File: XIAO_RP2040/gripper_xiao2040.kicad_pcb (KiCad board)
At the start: 2 copper layers, 41 x 48 mm, 18 parts, among them J1 GoFa IO, J2 VGoFa, J3 Servo, J4 Magnet, J5 Conn_01x04, U1 XIAO-RP2040-DIP, U2 HCPL-2631

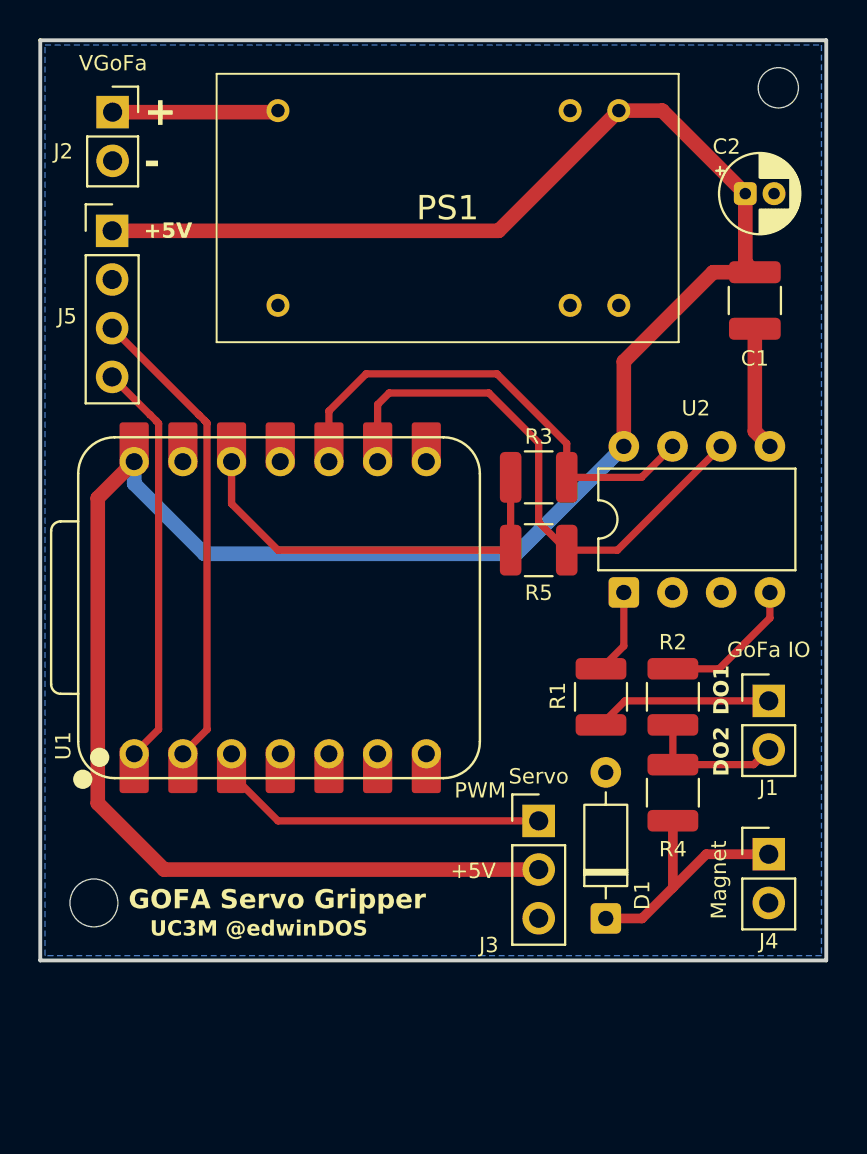
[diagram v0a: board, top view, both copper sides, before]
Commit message: PCB design complete and built. Arduino code still testing
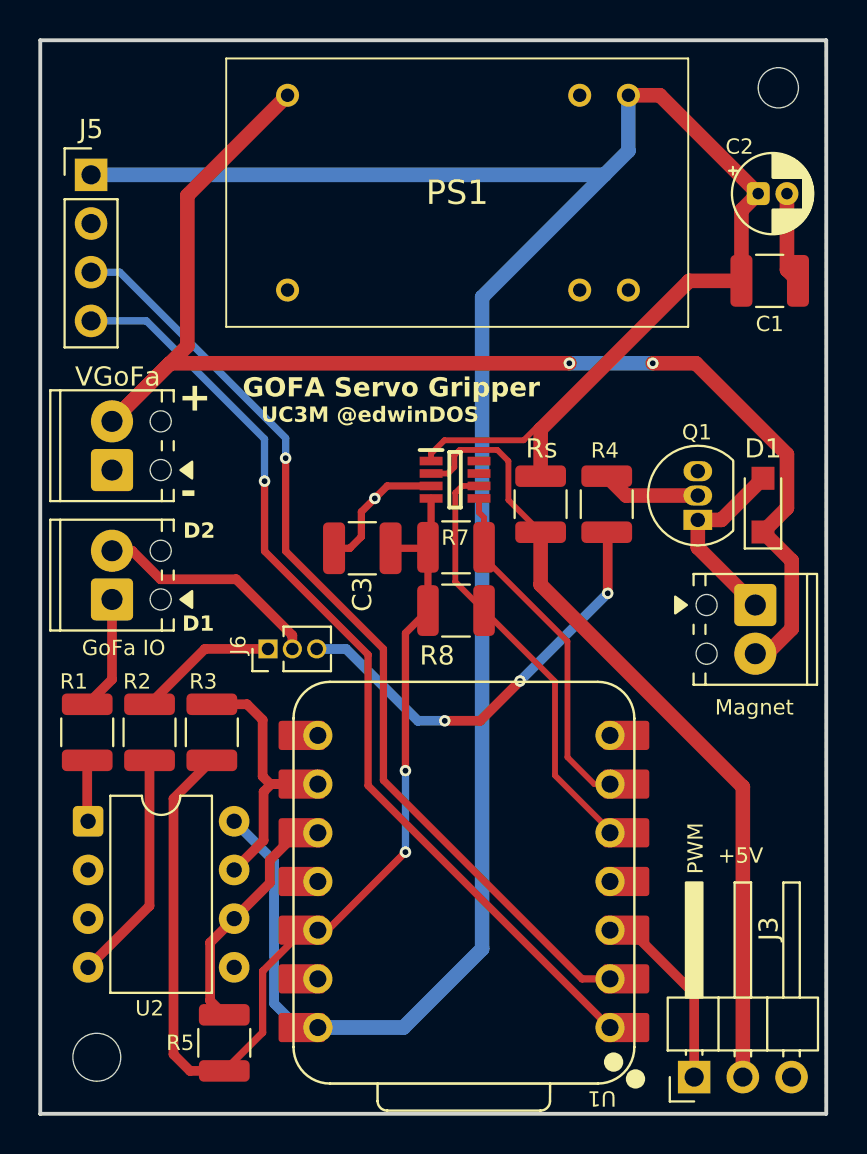
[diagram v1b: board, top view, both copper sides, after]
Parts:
- added C3: C, Capacitor_SMD:C_1210_3225Metric, F.Cu at (137.8, 103.5)
- added IC1: INA236BIDDFR, User:SOT65P280X110-8N, F.Cu at (142.6, 99.9)
- added J6: Jumper, Connector_PinHeader_1.27mm:PinHeader_1x03_P1.27mm_Vertical, F.Cu at (132.9, 108.8)
- added Q1: BC237, Package_TO_SOT_THT:TO-92_Inline, F.Cu at (155.3, 102.0)
- added R7: R, Resistor_SMD:R_1210_3225Metric, F.Cu at (142.7, 103.5)
- added R8: R, Resistor_SMD:R_1210_3225Metric, F.Cu at (142.7, 106.8)
- added Rs: R, Resistor_SMD:R_1210_3225Metric, F.Cu at (147.1, 101.2)
- D1: footprint Diode_THT:D_DO-35_SOD27_P7.62mm_Horizontal -> Diode_SMD:Nexperia_CFP3_SOD-123W
- J1, J4: footprint Connector_PinHeader_2.54mm:PinHeader_1x02_P2.54mm_Vertical -> TerminalBlock_Phoenix:TerminalBlock_Phoenix_MPT-0,5-2-2.54_1x02_P2.54mm_Horizontal
- J2: footprint Connector_PinSocket_2.54mm:PinSocket_1x02_P2.54mm_Vertical -> TerminalBlock_Phoenix:TerminalBlock_Phoenix_MPT-0,5-2-2.54_1x02_P2.54mm_Horizontal
- J3: footprint Connector_PinHeader_2.54mm:PinHeader_1x03_P2.54mm_Vertical -> Connector_PinHeader_2.54mm:PinHeader_1x03_P2.54mm_Horizontal
- R4: value R -> 4K7
- moved J1 34.7 mm to (124.7, 106.2), turned to 90 degrees
- moved R5 30.5 mm to (130.6, 129.3), turned to 90 degrees
- moved U2 30.4 mm to (123.5, 117.7), turned to 0 degrees
- moved R2 27.4 mm to (126.7, 113.1), turned to 90 degrees
- moved R1 26.9 mm to (123.5, 113.1), turned to -90 degrees
- moved D1 23.1 mm to (158.7, 101.2)
- moved R3 21.6 mm to (129.9, 113.1), turned to 90 degrees
- moved J2 18.7 mm to (124.7, 99.4), turned to 90 degrees
- moved U1 17.2 mm to (143.1, 120.9), turned to 180 degrees
- moved J3 15.6 mm to (155.1, 131.1), turned to 90 degrees
- moved R4 15.4 mm to (150.6, 101.2), turned to 90 degrees
- moved J4 13.0 mm to (158.3, 106.5), turned to -90 degrees
- moved REF** 8.05 mm to (124.0, 130.1)
- moved J5 3.12 mm to (123.7, 84.0)
- moved C1 1.29 mm to (159.1, 89.5), turned to 0 degrees
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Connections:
- D1 pad 1: Net-(D1-K) -> /VGoFa
- D1 pad 2: GND -> Net-(D1-A)
- J2 pad 1: /Vcc -> GND
- J2 pad 2: GND -> /VGoFa
- J3 pad 2: +5V -> /Vsensed
- J4 pad 1: Net-(D1-K) -> Net-(D1-A)
- J4 pad 2: GND -> /VGoFa
- PS1 pad 16: /Vcc -> /VGoFa
- R2 pad 2: /DO2 -> Net-(J6-Pin_1)
- R4 pad 1: /DO2 -> Net-(J6-Pin_3)
- R4 pad 2: Net-(D1-K) -> Net-(Q1-B)
- U1 pad 10: /do1_coupled -> /do2_coupled
- U1 pad 5: unconnected-(U1-GPIO6/SDA-Pad5) -> /SDA
- U1 pad 6: unconnected-(U1-GPIO7/SCL-Pad6) -> /SCL
- U1 pad 9: /do2_coupled -> /do1_coupled
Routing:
- net /VGoFa: track 0.00 -> 72.3 mm, vias 0 -> 2
- net /Vsensed: track 0.00 -> 42.3 mm
- net /+3V: track 21.6 -> 56.7 mm, vias 0 -> 2
- net /A0: track 22.3 -> 49.8 mm, vias 0 -> 1
- net /D2: track 25.9 -> 49.8 mm, vias 0 -> 1
- net Net-(J6-Pin_3): track 0.00 -> 22.7 mm, vias 0 -> 3
- net /SDA: track 0.00 -> 22.5 mm
- net /SCL: track 0.00 -> 18.2 mm
- net Net-(D1-K): track 16.6 -> 0.00 mm
- net /do2_coupled: track 29.2 -> 13.5 mm
- net Net-(D1-A): track 0.00 -> 10.2 mm
- net +5V: track 128.5 -> 138.7 mm
- net /Vcc: track 8.66 -> 0.00 mm
- net /PWM: track 18.1 -> 10.1 mm
- net /do1_coupled: track 24.5 -> 16.6 mm
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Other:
- board size 41 x 48 mm -> 41 x 56 mm
- board text added: "D1"
- board text added: "D2"
- board text removed: "DO1"
- board text removed: "DO2"
